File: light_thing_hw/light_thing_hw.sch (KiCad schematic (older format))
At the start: 58 parts, among them J1 CONNECTORS, J2 Li-Ion Battery, J3 ADDR_LED_PANEL_1_CONNECTORS, J4 ADDR_LED_PANEL_2_CONNECTORS, J5 MIC_CONN, Q1 MMBF170, Q2 BSS83P, SW1 ST_USER_BUTTON1, SW2 ST_RESET_BUTTON, U1 BC832-V1, U2 LSM6DS3, U3 MCP73833T-FCI_UN, U4 LMR62421XMF, U5 LP38511MRX-ADJ_NOPB, U5A1 STM32L452RETx

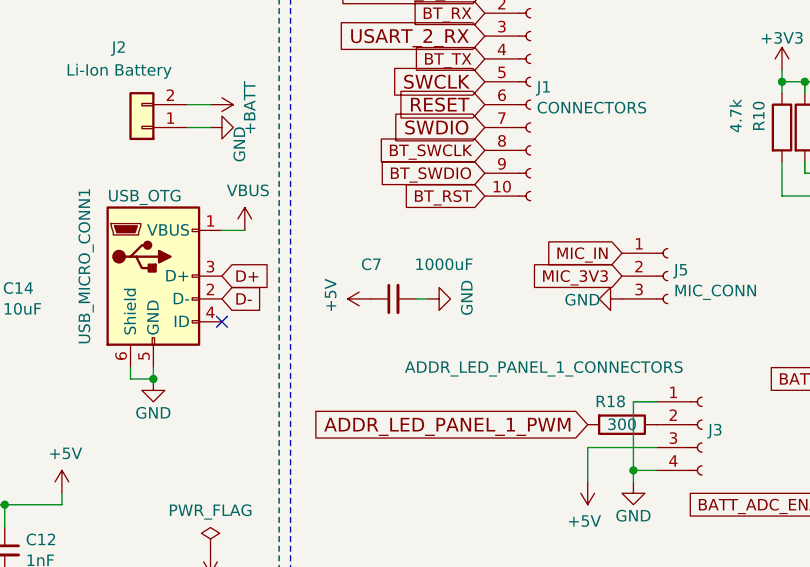
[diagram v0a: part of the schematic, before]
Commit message: hw updates. sent to print
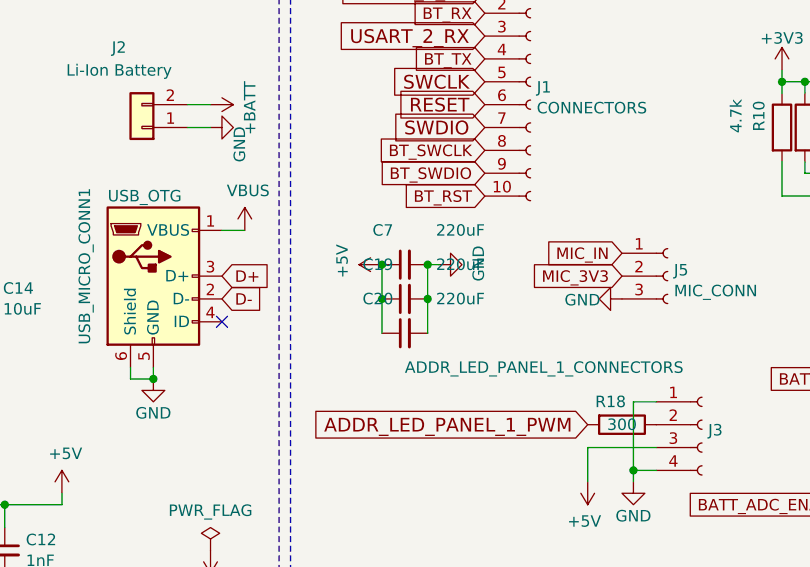
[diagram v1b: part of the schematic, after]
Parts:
- added C19, C20: 220uF, Capacitor_SMD:C_0603_1608Metric_Pad1.05x0.95mm_HandSolder, symbol Device:C_Small
- C7: value 1000uF -> 220uF
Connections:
- net +5V: now also C19.1, C20.1
- net GND: now also C19.2, C20.2
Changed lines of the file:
@@
 I2C2_SDA
-$Comp
-L Device:C_Small C7
-U 1 1 5ED59C90
-P 4500 3200
-F 0 "C7" V 4650 3250 50  0000 L CNN
-F 1 "1000uF" V 4650 2850 50  0000 L CNN
-F 2 "Capacitor_SMD:C_0603_1608Metric_Pad1.05x0.95mm_HandSolder" H 4500 3200 50  0001 C CNN
-F 3 "~" H 4500 3200 50  0001 C CNN
-	1    4500 3200
-	0    -1   -1   0
-$EndComp
 $Comp
 L power:GND #PWR08
 U 1 1 5ED59DA5
-P 4650 3200
-F 0 "#PWR08" H 4650 2950 50  0001 C CNN
-F 1 "GND" H 4655 3027 50  0000 C CNN
-F 2 "" H 4650 3200 50  0001 C CNN
-F 3 "" H 4650 3200 50  0001 C CNN
-	1    4650 3200
+P 4700 3050
+F 0 "#PWR08" H 4700 2800 50  0001 C CNN
+F 1 "GND" H 4705 2877 50  0000 C CNN
+F 2 "" H 4700 3050 50  0001 C CNN
+F 3 "" H 4700 3050 50  0001 C CNN
+	1    4700 3050
 	0    -1   -1   0
 $EndComp
 Wire Wire Line
-	4650 3200 4600 3200
+	4700 3050 4650 3050
 $Comp
 L power:GND #PWR016
@@
 L power:+5V #PWR0113
 U 1 1 5F0C7F22
-P 4400 3200
-F 0 "#PWR0113" H 4400 3050 50  0001 C CNN
-F 1 "+5V" H 4415 3373 50  0000 C CNN
-F 2 "" H 4400 3200 50  0001 C CNN
-F 3 "" H 4400 3200 50  0001 C CNN
-	1    4400 3200
+P 4450 3050
+F 0 "#PWR0113" H 4450 2900 50  0001 C CNN
+F 1 "+5V" H 4465 3223 50  0000 C CNN
+F 2 "" H 4450 3050 50  0001 C CNN
+F 3 "" H 4450 3050 50  0001 C CNN
+	1    4450 3050
 	0    -1   -1   0
 $EndComp
@@
 Text GLabel 5500 3100 0    50   Input ~ 0
 MIC_3V3
+$Comp
+L Device:C_Small C19
+U 1 1 5F158191
+P 4550 3200
+F 0 "C19" V 4700 3250 50  0000 L CNN
+F 1 "220uF" V 4700 2850 50  0000 L CNN
+F 2 "Capacitor_SMD:C_0603_1608Metric_Pad1.05x0.95mm_HandSolder" H 4550 3200 50  0001 C CNN
+F 3 "~" H 4550 3200 50  0001 C CNN
+	1    4550 3200
+	0    -1   -1   0
+$EndComp
+$Comp
+L Device:C_Small C7
+U 1 1 5F1706C5
+P 4550 3050
+F 0 "C7" V 4700 3100 50  0000 L CNN
+F 1 "220uF" V 4700 2700 50  0000 L CNN
+F 2 "Capacitor_SMD:C_0603_1608Metric_Pad1.05x0.95mm_HandSolder" H 4550 3050 50  0001 C CNN
+F 3 "~" H 4550 3050 50  0001 C CNN
+	1    4550 3050
+	0    -1   -1   0
+$EndComp
+$Comp
+L Device:C_Small C20
+U 1 1 5F17C8D1
+P 4550 3350
+F 0 "C20" V 4700 3400 50  0000 L CNN
+F 1 "220uF" V 4700 3000 50  0000 L CNN
+F 2 "Capacitor_SMD:C_0603_1608Metric_Pad1.05x0.95mm_HandSolder" H 4550 3350 50  0001 C CNN
+F 3 "~" H 4550 3350 50  0001 C CNN
+	1    4550 3350
+	0    -1   -1   0
+$EndComp
+Wire Wire Line
+	4450 3200 4450 3050
+Connection ~ 4450 3050
+Wire Wire Line
+	4450 3200 4450 3350
+Connection ~ 4450 3200
+Wire Wire Line
+	4650 3350 4650 3200
+Wire Wire Line
+	4650 3200 4650 3050
+Connection ~ 4650 3200
+Connection ~ 4650 3050
 $EndSCHEMATC
